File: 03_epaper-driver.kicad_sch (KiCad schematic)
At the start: 21 parts, among them J6 FFC2B28-24-G, Q4 BSS138

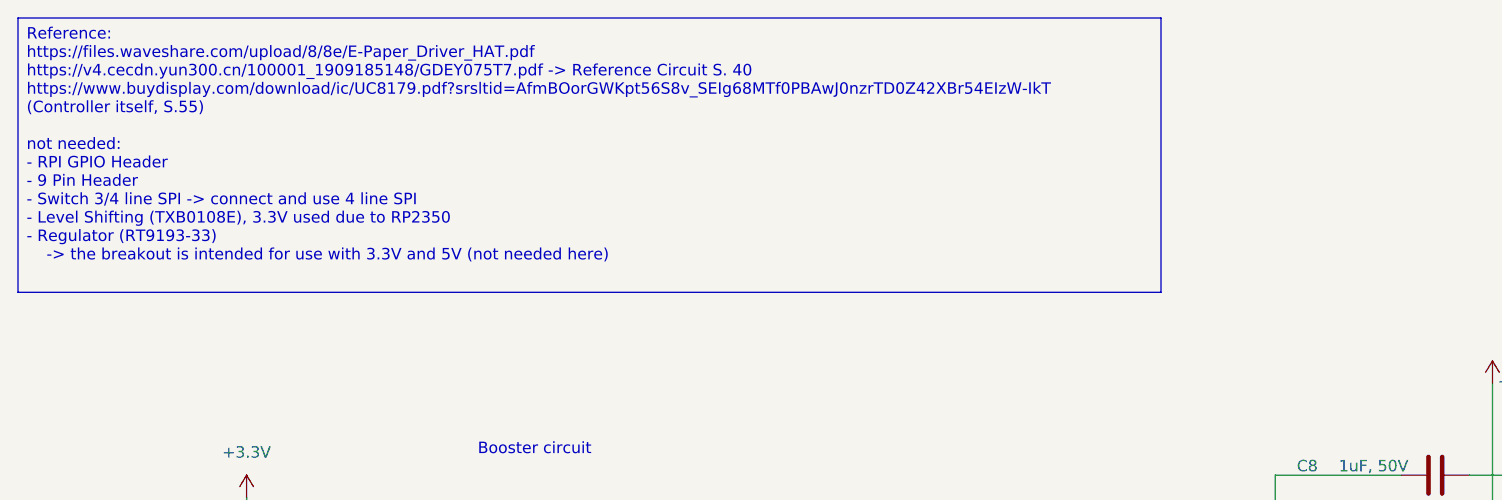
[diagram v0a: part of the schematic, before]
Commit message: Reworked the PCB after review
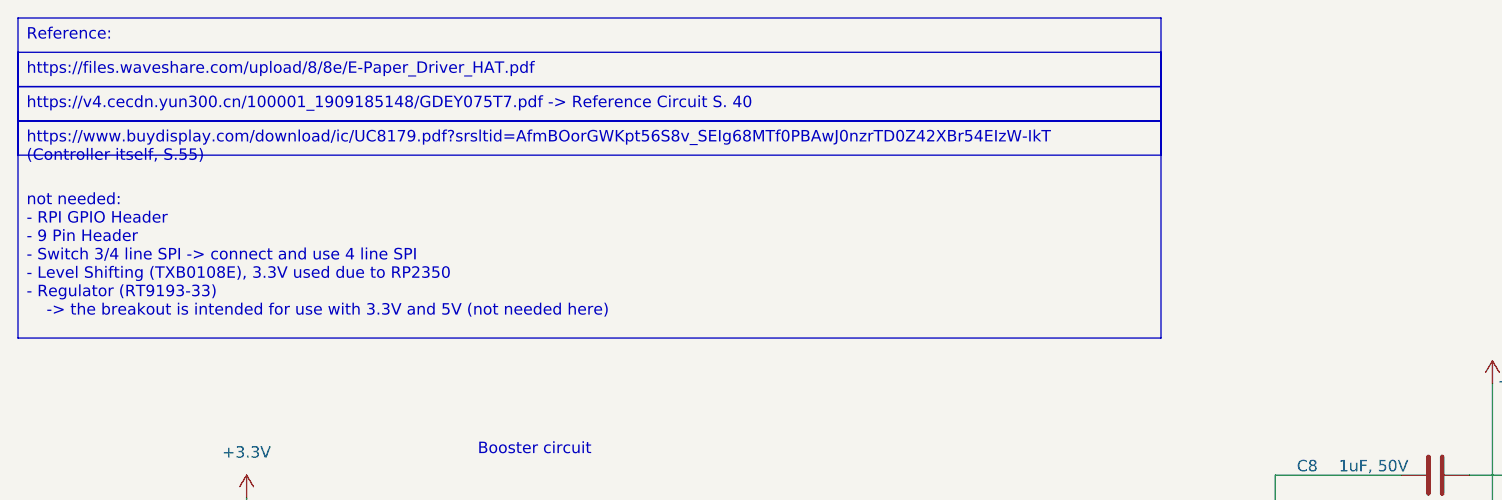
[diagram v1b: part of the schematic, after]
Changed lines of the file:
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@@
+		)
+	)
+	(text_box "https://files.waveshare.com/upload/8/8e/E-Paper_Driver_HAT.pdf"
+		(exclude_from_sim no)
+		(at 12.7 16.51 0)
+		(size 127 3.81)
+		(margins 0.9525 0.9525 0.9525 0.9525)
+		(stroke
+			(width 0)
+			(type solid)
+		)
+		(fill
+			(type none)
+		)
+		(effects
+			(font
+				(size 1.27 1.27)
+			)
+			(justify left top)
+			(href "https://files.waveshare.com/upload/8/8e/E-Paper_Driver_HAT.pdf")
 		)
 	)
@@
 		)
 	)
+	(text_box "https://v4.cecdn.yun300.cn/100001_1909185148/GDEY075T7.pdf -> Reference Circuit S. 40"
+		(exclude_from_sim no)
+		(at 12.7 20.32 0)
+		(size 127 3.81)
+		(margins 0.9525 0.9525 0.9525 0.9525)
+		(stroke
+			(width 0)
+			(type solid)
+		)
+		(fill
+			(type none)
+		)
+		(effects
+			(font
+				(size 1.27 1.27)
+			)
+			(justify left top)
+			(href "https://v4.cecdn.yun300.cn/100001_1909185148/GDEY075T7.pdf")
+		)
+	)
 	(text_box "Needs testing on the finished PCB if 4.7uF or 10uF"
 		(exclude_from_sim no)
 		(at 15.24 82.55 0)
 		(size 17.78 8.89)
+		(margins 0.9525 0.9525 0.9525 0.9525)
+		(stroke
+			(width 0)
+			(type solid)
+		)
+		(fill
+			(type none)
+		)
+		(effects
+			(font
+				(size 1.27 1.27)
+			)
+			(justify left top)
+		)
+	)
+	(text_box "https://www.buydisplay.com/download/ic/UC8179.pdf?srsltid=AfmBOorGWKpt56S8v_SEIg68MTf0PBAwJ0nzrTD0Z42XBr54EIzW-IkT (Controller itself, S.55)"
+		(exclude_from_sim no)
+		(at 12.7 24.13 0)
+		(size 127 3.81)
 		(margins 0.9525 0.9525 0.9525 0.9525)
 		(stroke
@@
 		)
 	)
-	(text_box "Reference:\nhttps://files.waveshare.com/upload/8/8e/E-Paper_Driver_HAT.pdf\nhttps://v4.cecdn.yun300.cn/100001_1909185148/GDEY075T7.pdf -> Reference Circuit S. 40\nhttps://www.buydisplay.com/download/ic/UC8179.pdf?srsltid=AfmBOorGWKpt56S8v_SEIg68MTf0PBAwJ0nzrTD0Z42XBr54EIzW-IkT (Controller itself, S.55)\n\nnot needed:\n- RPI GPIO Header\n- 9 Pin Header\n- Switch 3/4 line SPI -> connect and use 4 line SPI\n- Level Shifting (TXB0108E), 3.3V used due to RP2350\n- Regulator (RT9193-33) \n	-> the breakout is intended for use with 3.3V and 5V (not needed here)"
+	(text_box "Reference:\n\n\n\n\n\n\n\n\nnot needed:\n- RPI GPIO Header\n- 9 Pin Header\n- Switch 3/4 line SPI -> connect and use 4 line SPI\n- Level Shifting (TXB0108E), 3.3V used due to RP2350\n- Regulator (RT9193-33) \n	-> the breakout is intended for use with 3.3V and 5V (not needed here)"
 		(exclude_from_sim no)
 		(at 12.7 12.7 0)
-		(size 127 30.48)
+		(size 127 35.56)
 		(margins 0.9525 0.9525 0.9525 0.9525)
 		(stroke
@@
 			)
 			(justify left top)
-			(href "https://files.waveshare.com/upload/8/8e/E-Paper_Driver_HAT.pdf")
 		)
 	)
